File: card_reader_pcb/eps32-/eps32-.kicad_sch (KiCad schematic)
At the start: 27 parts, among them J1 Screw_Terminal_01x02, J2 Conn_01x08, U1 PPSM82916VCER, U2 ESP32-WROOM-32E

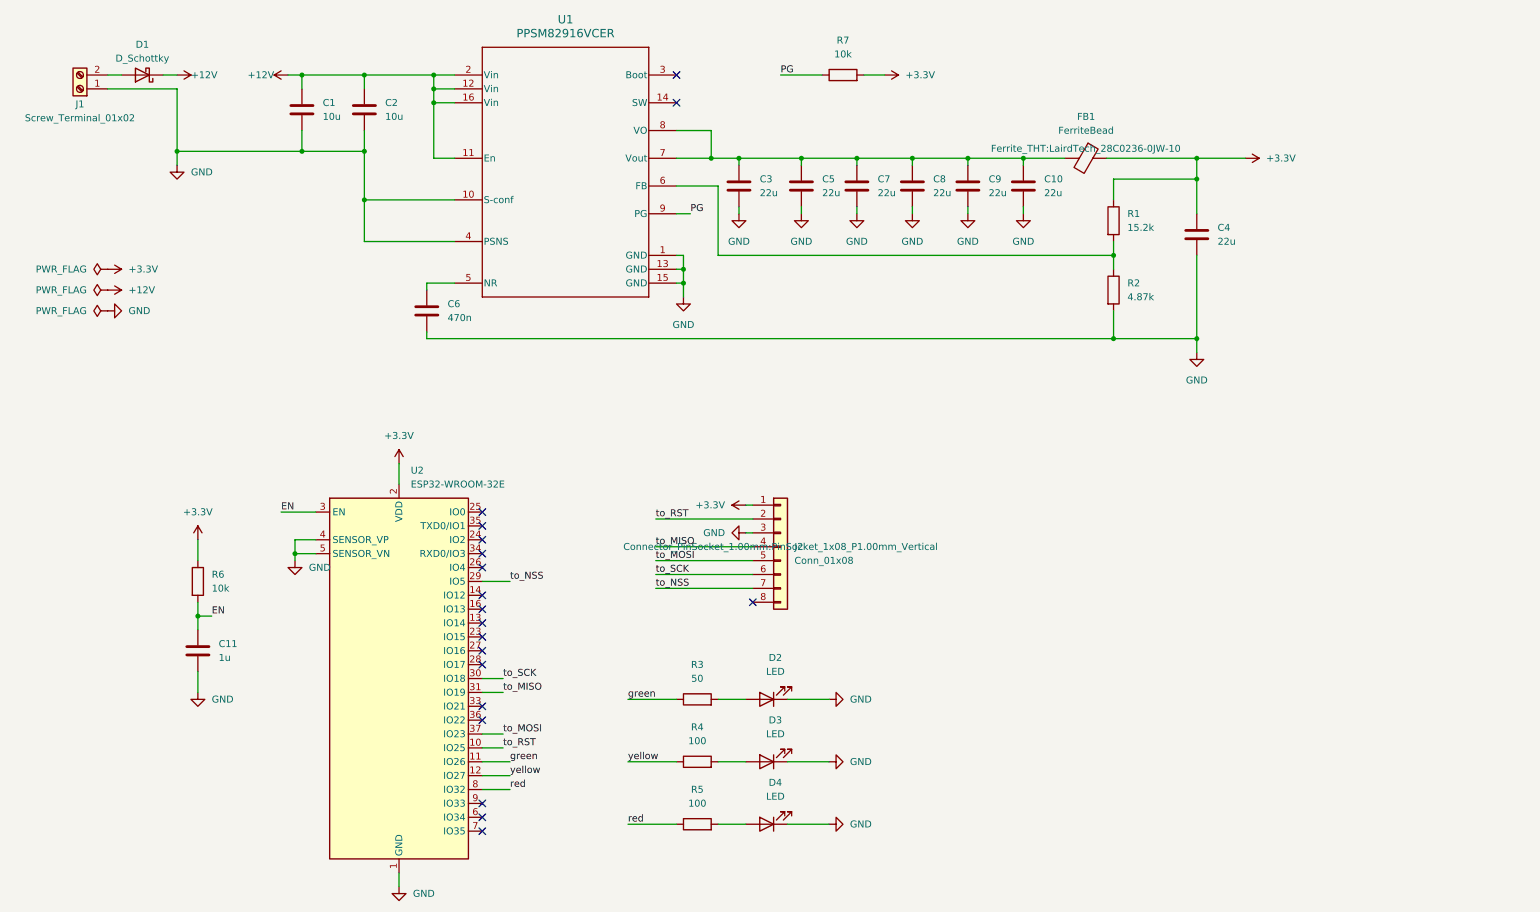
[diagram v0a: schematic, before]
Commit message: Add files via upload
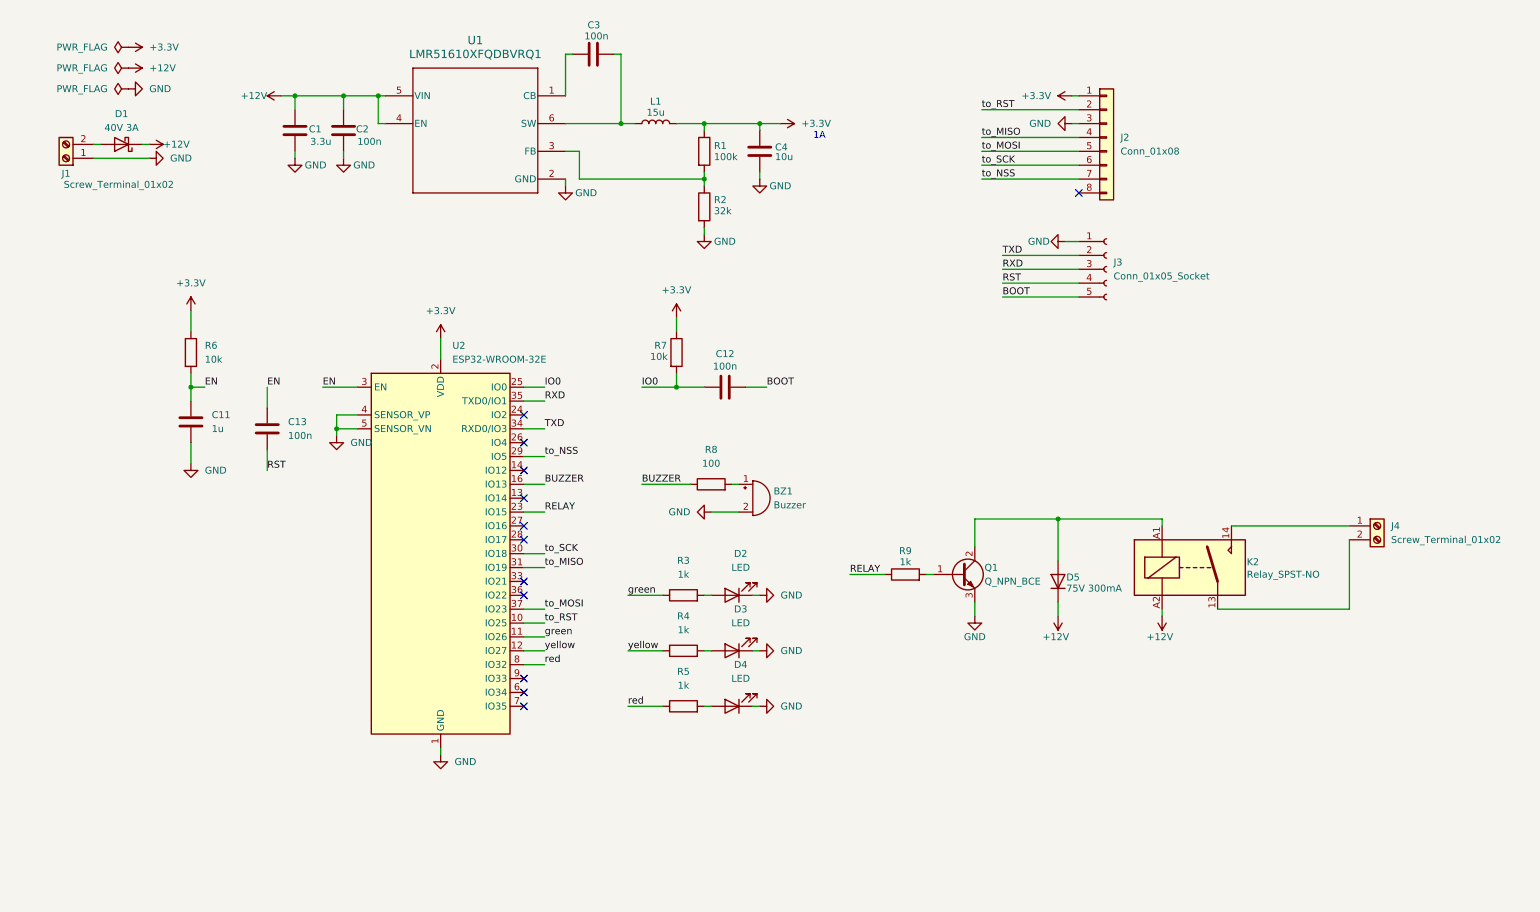
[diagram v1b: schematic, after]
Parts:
- removed C10, C5, C7, C8, C9: 22u, Capacitor_SMD:CP_Elec_4x5.3, symbol Device:C
- removed C6: 470n, Capacitor_SMD:CP_Elec_4x3, symbol Device:C
- removed FB1: FerriteBead, Ferrite_THT:LairdTech_28C0236-0JW-10, symbol Device:FerriteBead
- removed U1: PPSM82916VCER, PPSM82916VCER:VCE0016A-MFG, symbol TPSM82916:PPSM82916VCER
- added BZ1: Buzzer, Buzzer_Beeper:Buzzer_TDK_PS1240P02BT_D12.2mm_H6.5mm, symbol Device:Buzzer
- added C12, C13: 100n, Capacitor_SMD:C_0201_0603Metric, symbol Device:C
- added D5: 75V 300mA, Diode_SMD:D_0201_0603Metric, symbol Device:D
- added J3: Conn_01x05_Socket, Connector_PinHeader_1.00mm:PinHeader_1x05_P1.00mm_Vertical, symbol Connector:Conn_01x05_Socket
- added J4: Screw_Terminal_01x02, TerminalBlock:TerminalBlock_MaiXu_MX126-5.0-02P_1x02_P5.00mm, symbol Connector:Screw_Terminal_01x02
- added K2: Relay_SPST-NO, Relay_THT:Relay_SPST_Finder_32.21-x300, symbol Relay:Relay_SPST-NO
- added L1: 15u, Inductor_SMD:L_6.3x6.3_H3, symbol Device:L
- added Q1: Q_NPN_BCE, Package_TO_SOT_SMD:SOT-23, symbol Transistor_BJT:Q_NPN_BCE
- added R8: 100, Resistor_SMD:R_0603_1608Metric, symbol Device:R
- added R9: 1k, Resistor_SMD:R_0603_1608Metric, symbol Device:R
- added U1: LMR51610XFQDBVRQ1, LMR516:DBV0006A-IPC_C, symbol LMR51610XFQDBVRQ1:LMR51610XFQDBVRQ1
- C1: value 10u -> 3.3u; footprint Capacitor_SMD:CP_Elec_5x3 -> Capacitor_SMD:C_0201_0603Metric
- C11: footprint Capacitor_SMD:CP_Elec_4x5.4 -> Capacitor_SMD:C_0201_0603Metric
- C2: value 10u -> 100n; footprint Capacitor_SMD:CP_Elec_5x3 -> Capacitor_SMD:C_0201_0603Metric
- C3: value 22u -> 100n; footprint Capacitor_SMD:CP_Elec_4x5.3 -> Capacitor_SMD:C_0201_0603Metric
- C4: value 22u -> 10u; footprint Capacitor_SMD:CP_Elec_4x5.3 -> Capacitor_SMD:C_0201_0603Metric
- D1: value D_Schottky -> 40V 3A; footprint Diode_SMD:D_SMA -> Diode_SMD:D_0402_1005Metric
- R1: value 15.2k -> 100k
- R2: value 4.87k -> 32k
- R3: value 50 -> 1k
- R4, R5: value 100 -> 1k
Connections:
- net PG is gone; now on net +3.3V: R7.1
- net +12V: now also D5.1 (K), K2.A2, U1.4 (EN), U1.5 (VIN)
- net +3.3V: now also L1.2; no longer R7.2
- net EN: now also C13.1
- net GND: now also BZ1.2 (-), J3.1 (Pin_1), Q1.3 (E), U1.2 (GND); no longer C3.2
- net at C3.1: now also U1.1 (CB)
- net at R1.2, R2.1: now also U1.3 (FB)
- net BUZZER: now reaches U2.16 (IO13)
- net BUZZER: now also R8.1
- net RELAY: now reaches U2.23 (IO15)
- net RELAY: now also R9.1
- net IO0: now reaches U2.25 (IO0)
- net IO0: now also R7.2, C12.1
- net TXD: now reaches U2.34 (RXD0/IO3)
- net TXD: now also J3.2 (Pin_2)
- net RXD: now reaches U2.35 (TXD0/IO1)
- net RXD: now also J3.3 (Pin_3)
- new net: C3.2, L1.1, U1.6 (SW)
- new net: Q1.1 (B), R9.2
- new net: BZ1.1 (+), R8.2
- new net: D5.2 (A), K2.A1, Q1.2 (C)
- new net: J4.1 (Pin_1), K2.14
- new net: J4.2 (Pin_2), K2.13
- new net BOOT: C12.2, J3.5 (Pin_5)
- new net RST: C13.2, J3.4 (Pin_4)
- no-connect marks 19 -> 12
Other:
- note added: "1A"
- moved on the sheet: C11, D1, D2, D3, D4, J1, J2, R3, R4, R5, R6, U2
